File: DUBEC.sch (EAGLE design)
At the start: 46 parts

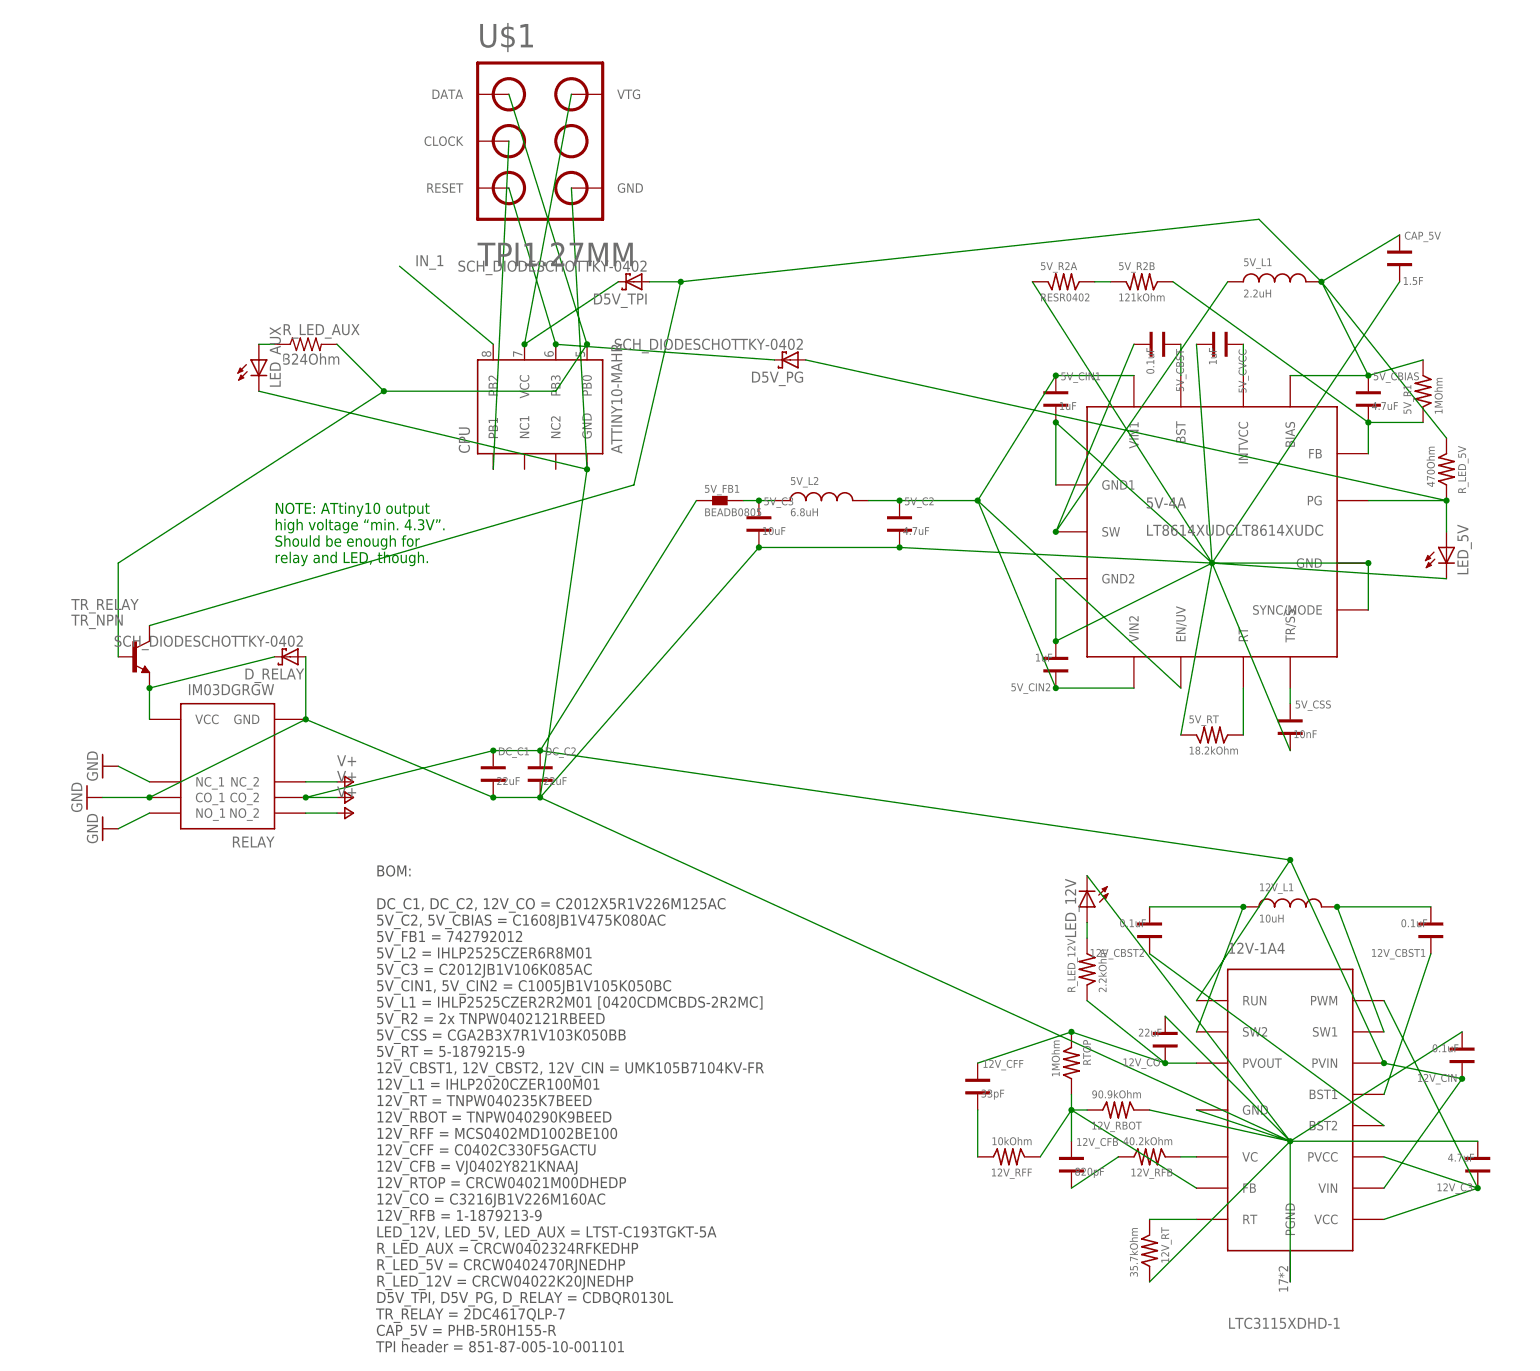
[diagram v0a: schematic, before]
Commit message: Flyback diode
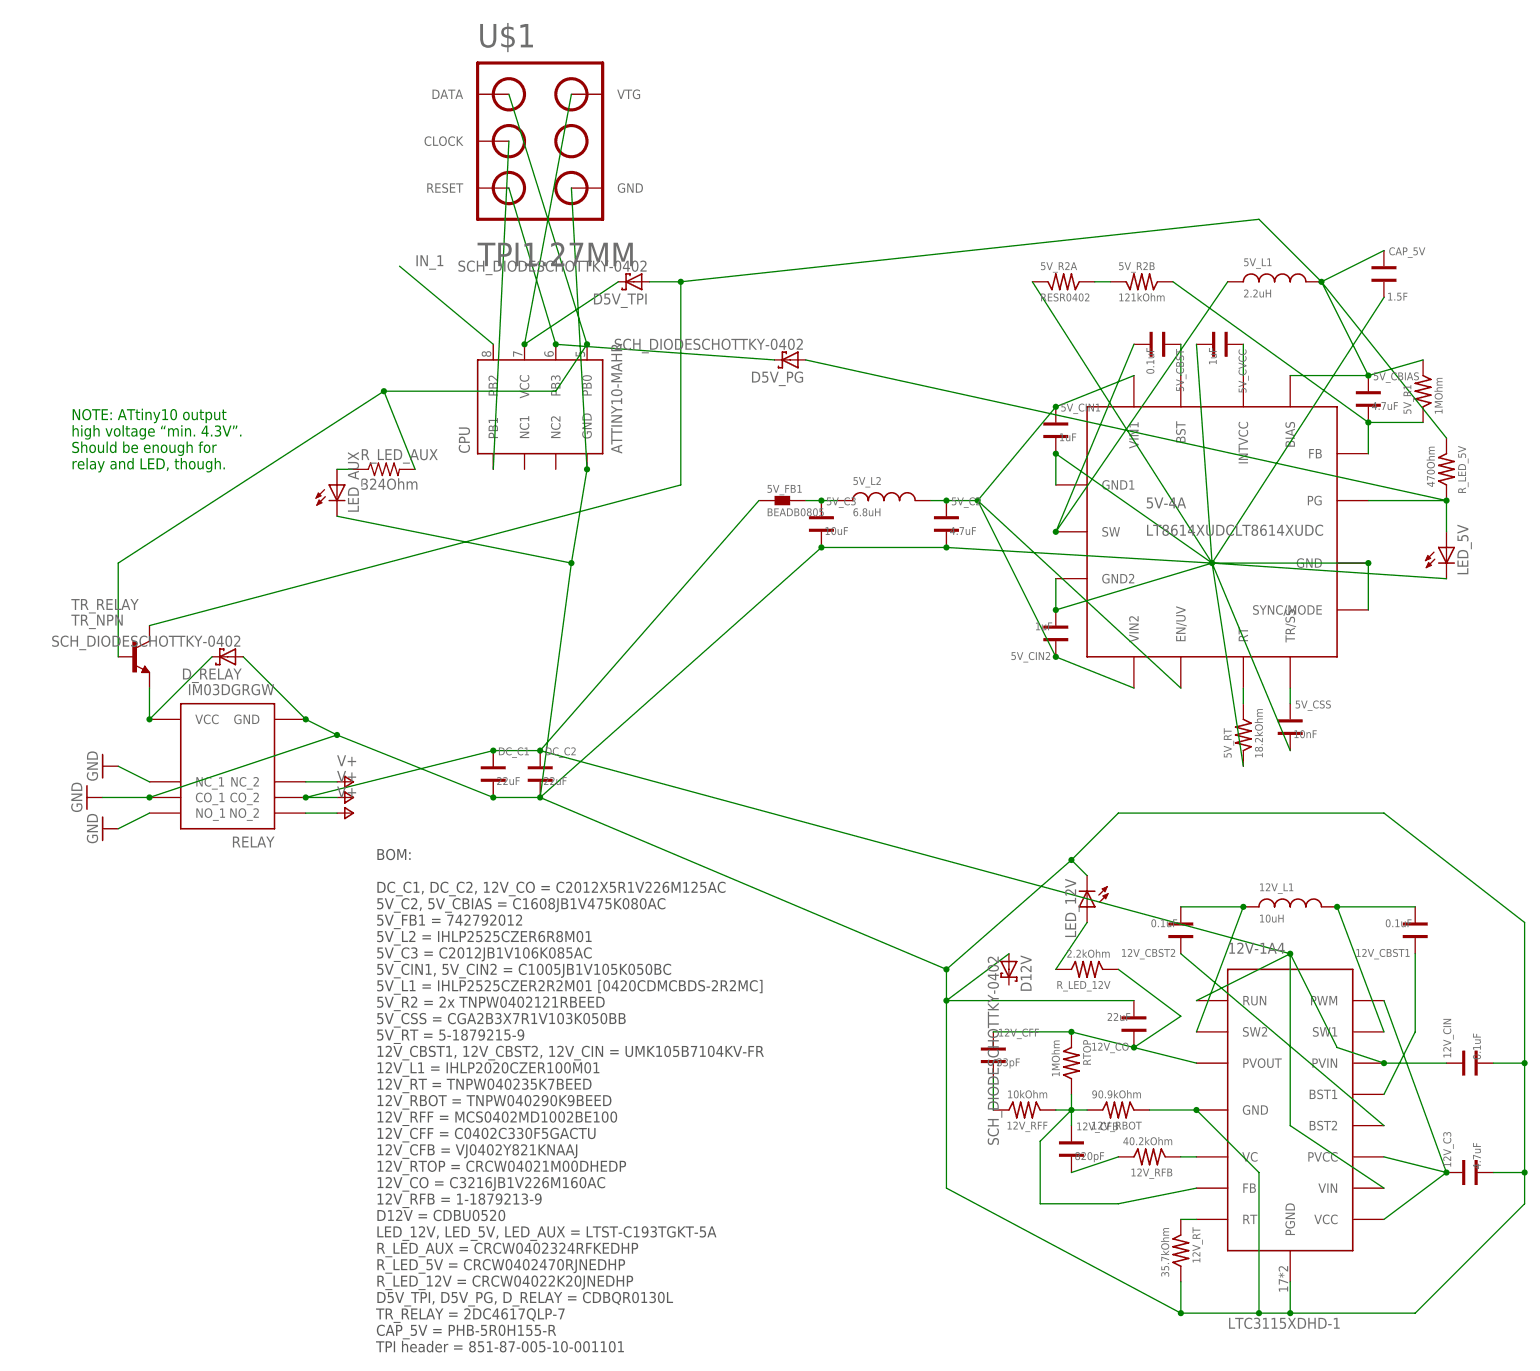
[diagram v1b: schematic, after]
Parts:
- added D12V: SCH_DIODESCHOTTKY-0402, dubec:SCH_DIODESCHOTTKY-0402
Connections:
- net GND: now also D12V.A
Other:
- moved on the sheet: 12V_C3, 12V_CBST1, 12V_CBST2, 12V_CFB, 12V_CFF, 12V_CIN, 12V_CO, 12V_RFF, 12V_RT, 5V_C2, 5V_C3, 5V_CIN1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
